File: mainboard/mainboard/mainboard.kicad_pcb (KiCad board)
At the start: 2 copper layers, 100 x 100 mm, 102 parts, among them IC501 SN74HCS138PWR, IC502 SN74HCS138PWR, IC503 SN74HCS138PWR, IC504 SN74HCS138PWR, IC505 SN74HCS151PWR, J1 Barrel_Jack_Switch, J201 Power LED connector, J202 Power button connector, J601 Connector 1, J602 Connector 6, J603 Connector 5, J604 Connector 4, J605 Connector 1, J606 Connector 3, J607 Connector 2, J608 I2C 2, J609 Conn_01x03_Female, J610 Conn_01x03_Female, J611 I2C 1, J612 I2C 3, J801 Micro_SD_Card, U201 RP2040, U301 LD1117S50TR_SOT223, U303 BD9D321EFJ, U304 BD9D321EFJ, U401 W25Q128JVS, U701 hs8836a, Y201 ECS-120-8-36-CGN-TR

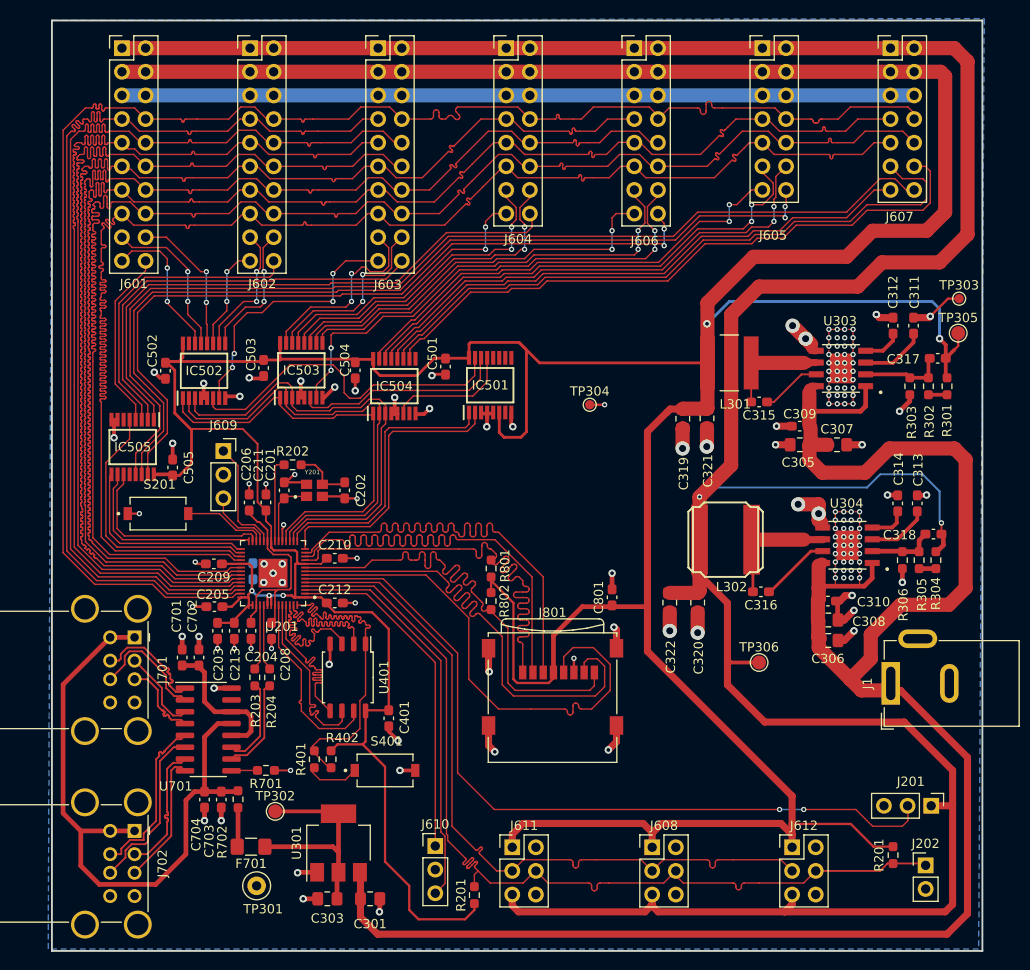
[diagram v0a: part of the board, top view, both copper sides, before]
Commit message: refactored mainboard schematic
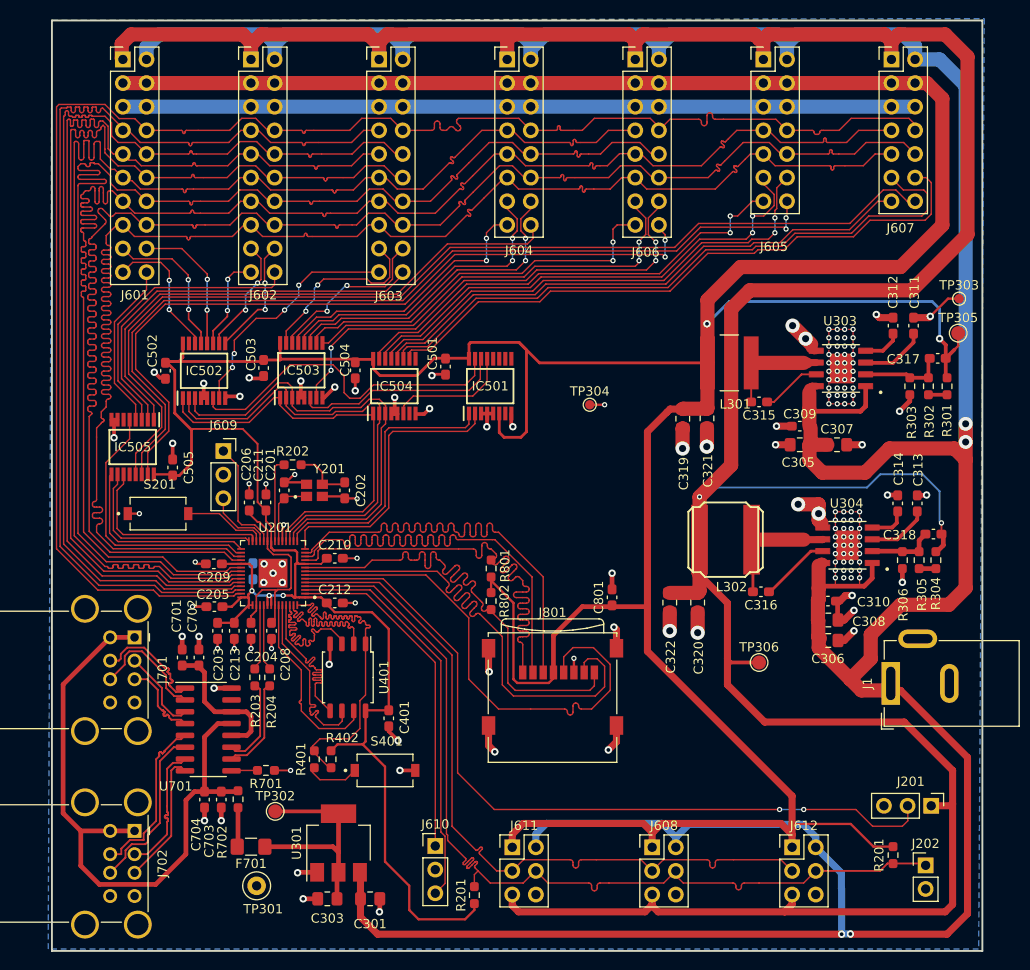
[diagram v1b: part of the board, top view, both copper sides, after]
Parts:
- IC501: value SN74HCS138PWR -> SN74HCS238PWR
- moved J604 1.22 mm to (71.9, 60.2)
- moved J605 1.22 mm to (99.5, 60.2)
- moved J606 1.22 mm to (85.7, 60.2)
- moved J607 1.22 mm to (113.2, 60.2)
- moved J601 1.22 mm to (30.6, 60.2)
- moved J602 1.22 mm to (44.4, 60.2)
- moved J603 1.22 mm to (58.2, 60.2)
- moved IC501 0.10 mm to (70.1, 95.3)
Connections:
- J601 pad 2: +5V_BUS -> VDC
- J602 pad 2: +5V_BUS -> VDC
- J603 pad 2: +5V_BUS -> VDC
- J604 pad 2: +5V_BUS -> VDC
- J605 pad 2: +5V_BUS -> VDC
- J606 pad 2: +5V_BUS -> VDC
- J607 pad 2: +5V_BUS -> VDC
- J608 pad 2: unconnected-(J608-Pin_2) -> VDC
- J611 pad 2: unconnected-(J611-Pin_2) -> VDC
- J612 pad 2: unconnected-(J612-Pin_2) -> VDC
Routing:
- net VDC: track 196.5 -> 393.8 mm, vias 0 -> 4
- net +5V_BUS: track 322.6 -> 345.1 mm
- net /Bus multiplexers & demultiplexers/BUS_CS4: track 28.6 -> 26.2 mm
- net /Bus multiplexers & demultiplexers/BUS_RE2: track 20.3 -> 18.4 mm
- net /Bus multiplexers & demultiplexers/BUS_CS3: track 14.5 -> 12.7 mm
- net /Connectors/BUS.D3: track 142.5 -> 144.3 mm
- net /Bus multiplexers & demultiplexers/BUS_RE1: track 14.6 -> 12.9 mm
- net /Bus multiplexers & demultiplexers/BUS_INT3: track 62.0 -> 60.4 mm
- net /Bus multiplexers & demultiplexers/BUS_INT2: track 45.6 -> 44.0 mm
- net /Bus multiplexers & demultiplexers/BUS_INT1: track 32.8 -> 31.2 mm
- net /Connectors/BUS.D1: track 174.9 -> 176.4 mm
- net /Connectors/BUS.D4: track 109.3 -> 110.8 mm
- net /Connectors/BUS.D5: track 109.2 -> 110.7 mm
- net /Bus multiplexers & demultiplexers/BUS_INT6: track 110.8 -> 109.4 mm
- net +3V3: track 539.0 -> 537.6 mm
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
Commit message: working on new pcb
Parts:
- removed C201, C202: 14p, Capacitor_SMD:C_0603_1608Metric_Pad1.08x0.95mm_HandSolder
- removed C204, C311, C313: 1u, Capacitor_SMD:C_0603_1608Metric_Pad1.08x0.95mm_HandSolder
- removed C206, C208, C209, C210, C211, C212, C213, C309, C310, C315, C316, C401, C501, C502, C503, C504, C505, C702, C704: 100n, Capacitor_SMD:C_0603_1608Metric_Pad1.08x0.95mm_HandSolder
- removed C301: 4.7u, Capacitor_SMD:C_0805_2012Metric_Pad1.18x1.45mm_HandSolder
- removed C303: 10uF, Capacitor_SMD:C_0805_2012Metric_Pad1.18x1.45mm_HandSolder
- removed C305, C306, C307, C308: 10u, Capacitor_SMD:C_0805_2012Metric_Pad1.18x1.45mm_HandSolder
- removed C312, C314: 3300p, Capacitor_SMD:C_0603_1608Metric_Pad1.08x0.95mm_HandSolder
- removed C317, C318: 22p, Capacitor_SMD:C_0603_1608Metric_Pad1.08x0.95mm_HandSolder
- removed C319, C320, C321, C322: 22u, Capacitor_SMD:C_0805_2012Metric_Pad1.18x1.45mm_HandSolder
- removed C701, C703: 4.7u, Capacitor_SMD:C_0603_1608Metric_Pad1.08x0.95mm_HandSolder
- removed C801: 10u, Capacitor_SMD:C_0603_1608Metric_Pad1.08x0.95mm_HandSolder
- removed F701: 500mA, Fuse:Fuse_1206_3216Metric_Pad1.42x1.75mm_HandSolder
- removed IC501: SN74HCS238PWR, footprints:SOP65P640X120-16N
- removed IC502, IC503, IC504: SN74HCS138PWR, footprints:SOP65P640X120-16N
- removed IC505: SN74HCS151PWR, footprints:SOP65P640X120-16N
- removed J201: Power LED connector, Connector_PinHeader_2.54mm:PinHeader_1x03_P2.54mm_Vertical
- removed J202: Power button connector, Connector_PinHeader_2.54mm:PinHeader_1x02_P2.54mm_Vertical
- removed J601: Connector 1, Connector_PinHeader_2.54mm:PinHeader_2x10_P2.54mm_Vertical
- removed J602: Connector 6, Connector_PinHeader_2.54mm:PinHeader_2x10_P2.54mm_Vertical
- removed J603: Connector 5, Connector_PinHeader_2.54mm:PinHeader_2x10_P2.54mm_Vertical
- removed J604: Connector 4, Connector_PinHeader_2.54mm:PinHeader_2x08_P2.54mm_Vertical
- removed J605: Connector 1, Connector_PinHeader_2.54mm:PinHeader_2x07_P2.54mm_Vertical
- removed J606: Connector 3, Connector_PinHeader_2.54mm:PinHeader_2x08_P2.54mm_Vertical
- removed J607: Connector 2, Connector_PinHeader_2.54mm:PinHeader_2x07_P2.54mm_Vertical
- removed J608: I2C 2, Connector_PinHeader_2.54mm:PinHeader_2x03_P2.54mm_Vertical
- removed J609: Conn_01x03_Female, Connector_PinSocket_2.54mm:PinSocket_1x03_P2.54mm_Vertical
- removed J610: Conn_01x03_Female, Connector_PinHeader_2.54mm:PinHeader_1x03_P2.54mm_Vertical
- removed J611: I2C 1, Connector_PinHeader_2.54mm:PinHeader_2x03_P2.54mm_Vertical
- removed J612: I2C 3, Connector_PinHeader_2.54mm:PinHeader_2x03_P2.54mm_Vertical
- removed J701, J702: ~, Connector_USB:USB_A_Wuerth_61400826021_Horizontal_Stacked
- removed J801: Micro_SD_Card, Connector_Card:microSD_HC_Wuerth_693072010801
- removed L301: 2.2u, footprints:IND_NR6028T4R7M
- removed L302: 3.3u, footprints:NRS8030
- removed R201 (x2), R402, R801, R802: 10k, Resistor_SMD:R_0603_1608Metric_Pad0.98x0.95mm_HandSolder
- removed R202, R401: 1k, Resistor_SMD:R_0603_1608Metric_Pad0.98x0.95mm_HandSolder
- removed R203, R204: 27.4R, Resistor_SMD:R_0603_1608Metric_Pad0.98x0.95mm_HandSolder
- removed R301: 68k, Resistor_SMD:R_0603_1608Metric_Pad0.98x0.95mm_HandSolder
- removed R302: 5.6k, Resistor_SMD:R_0603_1608Metric_Pad0.98x0.95mm_HandSolder
- removed R303, R306: 22k, Resistor_SMD:R_0603_1608Metric_Pad0.98x0.95mm_HandSolder
- removed R304: 120k, Resistor_SMD:R_0603_1608Metric_Pad0.98x0.95mm_HandSolder
- removed R305: 3.3k, Resistor_SMD:R_0603_1608Metric_Pad0.98x0.95mm_HandSolder
- removed R701: 100k, Resistor_SMD:R_0603_1608Metric_Pad0.98x0.95mm_HandSolder
- removed R702: 4.7, Resistor_SMD:R_0603_1608Metric_Pad0.98x0.95mm_HandSolder
- removed S201, S401: PTS636_SM43J_SMTR_LFS, footprints:SW_PTS636_SM43J_SMTR_LFS
- removed TP301: TestPoint, TestPoint:TestPoint_Loop_D1.80mm_Drill1.0mm_Beaded
- removed TP302, TP305, TP306: TestPoint, TestPoint:TestPoint_Pad_D1.5mm
- removed TP303, TP304: TestPoint, TestPoint:TestPoint_Pad_D1.0mm
- removed U201: RP2040, footprints:QFN40P700X700X90-57N
- removed U301: LD1117S50TR_SOT223, Package_TO_SOT_SMD:SOT-223-3_TabPin2
- removed U303, U304: BD9D321EFJ, footprints:SOIC127P600X100-9N
- removed U401: W25Q128JVS, Package_SO:SOIC-8_5.23x5.23mm_P1.27mm
- removed U701: hs8836a, Package_SO:SOP-16_3.9x9.9mm_P1.27mm
- removed Y201: ECS-120-8-36-CGN-TR, footprints:XTAL_ECS-120-8-36-CGN-TR
- added C1: 14p, Capacitor_SMD:C_0402_1005Metric_Pad0.74x0.62mm_HandSolder, F.Cu at (65.2, 57.8)
- added C10: 100n, Capacitor_SMD:C_0402_1005Metric_Pad0.74x0.62mm_HandSolder, F.Cu at (68.7, 63.8)
- added C11: 100n, Capacitor_SMD:C_0402_1005Metric_Pad0.74x0.62mm_HandSolder, F.Cu at (66.7, 69.1)
- added C12: 100n, Capacitor_SMD:C_0402_1005Metric_Pad0.74x0.62mm_HandSolder, F.Cu at (62.1, 71.9)
- added C13: 100n, Capacitor_SMD:C_0402_1005Metric_Pad0.74x0.62mm_HandSolder, F.Cu at (56.3, 69.2)
- added C14: 100n, Capacitor_SMD:C_0402_1005Metric_Pad0.74x0.62mm_HandSolder, F.Cu at (61.0, 71.2)
- added C15: 1u, Capacitor_SMD:C_0402_1005Metric_Pad0.74x0.62mm_HandSolder, F.Cu at (245.2, 61.9)
- added C16: 1u, Capacitor_SMD:C_0402_1005Metric_Pad0.74x0.62mm_HandSolder, F.Cu at (254.8, 63.9)
- added C17: 4.7u, Capacitor_SMD:C_0402_1005Metric_Pad0.74x0.62mm_HandSolder, F.Cu at (245.2, 60.0)
- added C18: 100pF, Capacitor_SMD:C_0402_1005Metric_Pad0.74x0.62mm_HandSolder, F.Cu at (245.2, 65.9)
- added C19: 100pF, Capacitor_SMD:C_0402_1005Metric_Pad0.74x0.62mm_HandSolder, F.Cu at (254.8, 65.9)
- added C2: 14p, Capacitor_SMD:C_0402_1005Metric_Pad0.74x0.62mm_HandSolder, F.Cu at (62.3, 54.4)
- added C20: 10uF, Capacitor_SMD:C_0402_1005Metric_Pad0.74x0.62mm_HandSolder, F.Cu at (245.2, 63.9)
- added C21: 2.2u, Capacitor_SMD:C_0402_1005Metric_Pad0.74x0.62mm_HandSolder, F.Cu at (254.8, 61.9)
- added C22: 2.2u, Capacitor_SMD:C_0402_1005Metric_Pad0.74x0.62mm_HandSolder, F.Cu at (254.8, 67.9)
- added C23: 10u, Capacitor_SMD:C_1206_3216Metric_Pad1.33x1.80mm_HandSolder, F.Cu at (134.1, 108.7)
- added C24: 10u, Capacitor_SMD:C_1206_3216Metric_Pad1.33x1.80mm_HandSolder, F.Cu at (117.0, 108.5)
- added C25: 10u, Capacitor_SMD:C_1206_3216Metric_Pad1.33x1.80mm_HandSolder, F.Cu at (131.4, 108.7)
- added C26: 10u, Capacitor_SMD:C_1206_3216Metric_Pad1.33x1.80mm_HandSolder, F.Cu at (114.3, 108.5)
- added C27: 100n, Capacitor_SMD:C_0402_1005Metric_Pad0.74x0.62mm_HandSolder, F.Cu at (136.0, 108.1)
- added C28: 100n, Capacitor_SMD:C_0402_1005Metric_Pad0.74x0.62mm_HandSolder, F.Cu at (118.9, 107.8)
- added C29: 1u, Capacitor_SMD:C_0402_1005Metric_Pad0.74x0.62mm_HandSolder, F.Cu at (144.3, 115.3)
- added C3: 1u, Capacitor_SMD:C_0402_1005Metric_Pad0.74x0.62mm_HandSolder, F.Cu at (58.7, 71.2)
- added C30: 3300p, Capacitor_SMD:C_0402_1005Metric_Pad0.74x0.62mm_HandSolder, F.Cu at (144.3, 114.2)
- added C31: 1u, Capacitor_SMD:C_0402_1005Metric_Pad0.74x0.62mm_HandSolder, F.Cu at (126.9, 115.2)
- added C32: 3300p, Capacitor_SMD:C_0402_1005Metric_Pad0.74x0.62mm_HandSolder, F.Cu at (126.9, 114.1)
- added C33: 100n, Capacitor_SMD:C_0402_1005Metric_Pad0.74x0.62mm_HandSolder, F.Cu at (135.0, 101.9)
- added C34: 100n, Capacitor_SMD:C_0402_1005Metric_Pad0.74x0.62mm_HandSolder, F.Cu at (119.5, 102.5)
- added C35: 22p, Capacitor_SMD:C_0402_1005Metric_Pad0.74x0.62mm_HandSolder, F.Cu at (140.3, 116.5)
- added C36: 22p, Capacitor_SMD:C_0402_1005Metric_Pad0.74x0.62mm_HandSolder, F.Cu at (123.2, 116.3)
- added C37: 22u, Capacitor_SMD:C_1206_3216Metric_Pad1.33x1.80mm_HandSolder, F.Cu at (144.7, 93.6)
- added C38: 22u, Capacitor_SMD:C_1206_3216Metric_Pad1.33x1.80mm_HandSolder, F.Cu at (127.6, 95.2)
- added C39: 22u, Capacitor_SMD:C_1206_3216Metric_Pad1.33x1.80mm_HandSolder, F.Cu at (144.7, 90.9)
- added C4: 100n, Capacitor_SMD:C_0402_1005Metric_Pad0.74x0.62mm_HandSolder, F.Cu at (57.5, 71.2)
- added C40: 22u, Capacitor_SMD:C_1206_3216Metric_Pad1.33x1.80mm_HandSolder, F.Cu at (127.6, 92.6)
- added C41: 4.7u, Capacitor_SMD:C_0402_1005Metric_Pad0.74x0.62mm_HandSolder, F.Cu at (40.0, 121.1)
- added C42: 100n, Capacitor_SMD:C_0402_1005Metric_Pad0.74x0.62mm_HandSolder, F.Cu at (40.0, 123.0)
- added C43: 4.7u, Capacitor_SMD:C_0402_1005Metric_Pad0.74x0.62mm_HandSolder, F.Cu at (40.0, 125.0)
- added C44: 1u, Capacitor_SMD:C_0402_1005Metric_Pad0.74x0.62mm_HandSolder, F.Cu at (60.6, 107.5)
- added C45: 100n, Capacitor_SMD:C_0402_1005Metric_Pad0.74x0.62mm_HandSolder, F.Cu at (70.0, 100.3)
- added C46: 100n, Capacitor_SMD:C_0402_1005Metric_Pad0.74x0.62mm_HandSolder, F.Cu at (69.3, 104.8)
- added C47: 1u, Capacitor_SMD:C_0402_1005Metric_Pad0.74x0.62mm_HandSolder, F.Cu at (61.8, 107.5)
- added C48: 100n, Capacitor_SMD:C_0402_1005Metric_Pad0.74x0.62mm_HandSolder, F.Cu at (58.3, 104.7)
- added C49: 100n, Capacitor_SMD:C_0402_1005Metric_Pad0.74x0.62mm_HandSolder, F.Cu at (66.6, 108.5)
- added C5: 1u, Capacitor_SMD:C_0402_1005Metric_Pad0.74x0.62mm_HandSolder, F.Cu at (59.8, 71.2)
- added C50: 100n, Capacitor_SMD:C_0402_1005Metric_Pad0.74x0.62mm_HandSolder, F.Cu at (65.4, 108.5)
- added C51: 100n, Capacitor_SMD:C_0402_1005Metric_Pad0.74x0.62mm_HandSolder, F.Cu at (62.9, 94.0)
- added C52: 100n, Capacitor_SMD:C_0402_1005Metric_Pad0.74x0.62mm_HandSolder, F.Cu at (63.8, 107.8)
- added C53: 100n, Capacitor_SMD:C_0402_1005Metric_Pad0.74x0.62mm_HandSolder, F.Cu at (64.0, 94.0)
- added C54: 100n, Capacitor_SMD:C_0402_1005Metric_Pad0.74x0.62mm_HandSolder, F.Cu at (58.0, 100.0)
- added C55: 100n, Capacitor_SMD:C_0402_1005Metric_Pad0.74x0.62mm_HandSolder, F.Cu at (59.5, 107.5)
- added C56: 1u, Capacitor_SMD:C_0402_1005Metric_Pad0.74x0.62mm_HandSolder, F.Cu at (232.8, 103.5)
- added C57: 1u, Capacitor_SMD:C_0402_1005Metric_Pad0.74x0.62mm_HandSolder, F.Cu at (232.8, 97.6)
- added C58: 1u, Capacitor_SMD:C_0402_1005Metric_Pad0.74x0.62mm_HandSolder, F.Cu at (236.0, 95.6)
- added C59: 1u, Capacitor_SMD:C_0402_1005Metric_Pad0.74x0.62mm_HandSolder, F.Cu at (239.3, 97.6)
- added C6: 100n, Capacitor_SMD:C_0402_1005Metric_Pad0.74x0.62mm_HandSolder, F.Cu at (61.7, 57.7)
- added C60: 1u, Capacitor_SMD:C_0402_1005Metric_Pad0.74x0.62mm_HandSolder, F.Cu at (232.8, 101.5)
- added C61: 100n, Capacitor_SMD:C_0402_1005Metric_Pad0.74x0.62mm_HandSolder, F.Cu at (239.3, 99.6)
- added C62: 100n, Capacitor_SMD:C_0402_1005Metric_Pad0.74x0.62mm_HandSolder, F.Cu at (232.8, 95.6)
- added C63: 100n, Capacitor_SMD:C_0402_1005Metric_Pad0.74x0.62mm_HandSolder, F.Cu at (232.8, 99.6)
- added C64: 22u, Capacitor_SMD:C_0402_1005Metric_Pad0.74x0.62mm_HandSolder, F.Cu at (236.0, 103.5)
- added C65: 100n, Capacitor_SMD:C_0402_1005Metric_Pad0.74x0.62mm_HandSolder, F.Cu at (239.3, 95.6)
- added C66: 1u, Capacitor_SMD:C_0402_1005Metric_Pad0.74x0.62mm_HandSolder, F.Cu at (236.0, 97.6)
- added C67: 1u, Capacitor_SMD:C_0402_1005Metric_Pad0.74x0.62mm_HandSolder, F.Cu at (236.0, 99.6)
- added C68: 1u, Capacitor_SMD:C_0402_1005Metric_Pad0.74x0.62mm_HandSolder, F.Cu at (236.0, 101.5)
- added C69: 100n, Capacitor_SMD:C_0402_1005Metric_Pad0.74x0.62mm_HandSolder, F.Cu at (110.2, 97.4)
- added C7: 100n, Capacitor_SMD:C_0402_1005Metric_Pad0.74x0.62mm_HandSolder, F.Cu at (63.2, 72.5)
- added C70: 100n, Capacitor_SMD:C_0402_1005Metric_Pad0.74x0.62mm_HandSolder, F.Cu at (102.5, 98.7)
- added C71: 100n, Capacitor_SMD:C_0402_1005Metric_Pad0.74x0.62mm_HandSolder, F.Cu at (87.5, 92.2)
- added C72: 10u, Capacitor_SMD:C_0402_1005Metric_Pad0.74x0.62mm_HandSolder, F.Cu at (306.6, 64.0)
- added C72: 4.7u, Capacitor_SMD:C_0402_1005Metric_Pad0.74x0.62mm_HandSolder, F.Cu at (249.1, 43.9)
- added C73: 14p, Capacitor_SMD:C_0402_1005Metric_Pad0.74x0.62mm_HandSolder, F.Cu at (70.4, 92.8)
- added C73: 100n, Capacitor_SMD:C_0402_1005Metric_Pad0.74x0.62mm_HandSolder, F.Cu at (249.1, 45.8)
- added C74: 4.7u, Capacitor_SMD:C_0402_1005Metric_Pad0.74x0.62mm_HandSolder, F.Cu at (249.1, 47.8)
- added C74: 14p, Capacitor_SMD:C_0402_1005Metric_Pad0.74x0.62mm_HandSolder, F.Cu at (68.2, 90.5)
- added C75: 100n, Capacitor_SMD:C_0402_1005Metric_Pad0.74x0.62mm_HandSolder, F.Cu at (76.8, 113.0)
- added C76: 100n, Capacitor_SMD:C_0402_1005Metric_Pad0.74x0.62mm_HandSolder, F.Cu at (61.1, 81.4)
- added C77: 100n, Capacitor_SMD:C_0402_1005Metric_Pad0.74x0.62mm_HandSolder, F.Cu at (82.3, 77.7)
- added C78: 100n, Capacitor_SMD:C_0402_1005Metric_Pad0.74x0.62mm_HandSolder, F.Cu at (85.7, 85.5)
- added C8: 100n, Capacitor_SMD:C_0402_1005Metric_Pad0.74x0.62mm_HandSolder, F.Cu at (55.6, 63.8)
- added C9: 100n, Capacitor_SMD:C_0402_1005Metric_Pad0.74x0.62mm_HandSolder, F.Cu at (60.6, 57.7)
- added D1: LESD5D5.0CT1G, footprints:TVS_LESD5D5.0CT1G, F.Cu at (24.3, 121.2)
- added D10: LESD5D5.0CT1G, footprints:TVS_LESD5D5.0CT1G, F.Cu at (81.5, 131.1)
- added D10: LESD5D5.0CT1G, footprints:TVS_LESD5D5.0CT1G, F.Cu at (28.2, 128.3)
- added D11: LESD5D5.0CT1G, footprints:TVS_LESD5D5.0CT1G, F.Cu at (63.0, 123.4)
- added D11: WS2812B, LED_SMD:LED_WS2812B_PLCC4_5.0x5.0mm_P3.2mm, F.Cu at (298.4, 90.5)
- added D2: LESD5D5.0CT1G, footprints:TVS_LESD5D5.0CT1G, F.Cu at (59.1, 116.4)
- added D2: LESD5D5.0CT1G, footprints:TVS_LESD5D5.0CT1G, F.Cu at (24.3, 123.6)
- added D3: LESD5D5.0CT1G, footprints:TVS_LESD5D5.0CT1G, F.Cu at (83.1, 131.1)
- added D3: LESD5D5.0CT1G, footprints:TVS_LESD5D5.0CT1G, F.Cu at (24.3, 126.0)
- added D4: LESD5D5.0CT1G, footprints:TVS_LESD5D5.0CT1G, F.Cu at (59.1, 118.7)
- added D4: LESD5D5.0CT1G, footprints:TVS_LESD5D5.0CT1G, F.Cu at (24.3, 128.3)
- added D5: LESD5D5.0CT1G, footprints:TVS_LESD5D5.0CT1G, F.Cu at (24.3, 130.7)
- added D5: LESD5D5.0CT1G, footprints:TVS_LESD5D5.0CT1G, F.Cu at (63.0, 116.4)
- added D6: LESD5D5.0CT1G, footprints:TVS_LESD5D5.0CT1G, F.Cu at (24.3, 133.0)
- added D6: LESD5D5.0CT1G, footprints:TVS_LESD5D5.0CT1G, F.Cu at (59.1, 121.1)
- added D7: LESD5D5.0CT1G, footprints:TVS_LESD5D5.0CT1G, F.Cu at (28.2, 121.2)
- added D7: LESD5D5.0CT1G, footprints:TVS_LESD5D5.0CT1G, F.Cu at (63.0, 118.7)
- added D8: LESD5D5.0CT1G, footprints:TVS_LESD5D5.0CT1G, F.Cu at (59.1, 123.4)
- added D8: LESD5D5.0CT1G, footprints:TVS_LESD5D5.0CT1G, F.Cu at (28.2, 123.6)
- added D9: LESD5D5.0CT1G, footprints:TVS_LESD5D5.0CT1G, F.Cu at (28.2, 126.0)
- added D9: LESD5D5.0CT1G, footprints:TVS_LESD5D5.0CT1G, F.Cu at (63.0, 121.1)
- added IC1: SN74HCS151PWR, footprints:SOP65P640X120-16N, F.Cu at (99.1, 94.6)
- added IC2: SN74HCS151PWR, footprints:SOP65P640X120-16N, F.Cu at (106.7, 94.6)
- added IC3: SN74HCS138PWR, footprints:SOP65P640X120-16N, F.Cu at (91.4, 94.6)
- added IC4: SN74HCS138PWR, footprints:SOP65P640X120-16N, F.Cu at (80.0, 81.3)
- added IC5: SN74HCS138PWR, footprints:SOP65P640X120-16N, F.Cu at (80.0, 87.6)
- added J10: AudioJack4, Connector_Audio:Jack_3.5mm_PJ320D_Horizontal, F.Cu at (103.0, 126.4)
- added J11: AudioJack4, Connector_Audio:Jack_3.5mm_PJ320D_Horizontal, F.Cu at (115.4, 126.4)
- added J12: Conn_01x03_Female, Connector_PinHeader_2.54mm:PinHeader_1x03_P2.54mm_Vertical, F.Cu at (54.4, 54.1)
- added J13: Connector 16-bit, Connector_PinHeader_1.27mm:PinHeader_2x15_P1.27mm_Vertical_SMD, F.Cu at (83.8, 64.1)
- added J14: Connector A 8-bit, Connector_PinHeader_1.27mm:PinHeader_2x10_P1.27mm_Vertical_SMD, F.Cu at (102.2, 79.9)
- added J15: Connector B 8-bit, Connector_PinHeader_1.27mm:PinHeader_2x10_P1.27mm_Vertical_SMD, F.Cu at (102.2, 61.0)
- added J16: Connector A - 4 bit, Connector_PinHeader_1.27mm:PinHeader_2x08_P1.27mm_Vertical_SMD, F.Cu at (120.7, 78.7)
- added J17: Connector B - 4 bit, Connector_PinHeader_1.27mm:PinHeader_2x08_P1.27mm_Vertical_SMD, F.Cu at (120.5, 59.7)
- added J18: Connector A - 2 bit, Connector_PinHeader_1.27mm:PinHeader_2x05_P1.27mm_Vertical_SMD, F.Cu at (139.1, 76.8)
- added J19: Connector B - 2 bit, Connector_PinHeader_1.27mm:PinHeader_2x05_P1.27mm_Vertical_SMD, F.Cu at (139.1, 57.8)
- added J2: ~, Connector_USB:USB_A_Wuerth_61400826021_Horizontal_Stacked, F.Cu at (83.1, 135.0)
- added J3: ~, Connector_USB:USB_A_Wuerth_61400826021_Horizontal_Stacked, F.Cu at (62.9, 135.0)
- added J4: Micro_SD_Card, Connector_Card:microSD_HC_Wuerth_693072010801, F.Cu at (207.6, 139.6)
- added J5: I2C 2, Connector_PinHeader_2.54mm:PinHeader_2x03_P2.54mm_Vertical, F.Cu at (266.5, 61.3)
- added J6: Conn_01x03_Female, Connector_PinSocket_2.54mm:PinSocket_1x03_P2.54mm_Vertical, F.Cu at (58.8, 89.3)
- added J7: I2C 1, Connector_PinHeader_2.54mm:PinHeader_2x03_P2.54mm_Vertical, F.Cu at (273.7, 61.3)
- added J8: I2C 3, Connector_PinHeader_2.54mm:PinHeader_2x03_P2.54mm_Vertical, F.Cu at (280.9, 61.3)
- added J9: Conn_01x03_Female, Connector_PinHeader_2.54mm:PinHeader_1x03_P2.54mm_Vertical, F.Cu at (80.8, 105.7)
- added L1: 3.3u, footprints:NRS8030, F.Cu at (140.5, 99.3)
- added L2: 2.2u, footprints:IND_NR6028T4R7M, F.Cu at (123.6, 100.2)
- added R1: 1k, Resistor_SMD:R_0402_1005Metric_Pad0.72x0.64mm_HandSolder, F.Cu at (62.9, 56.1)
- added R10: 27.4R, Resistor_SMD:R_0402_1005Metric_Pad0.72x0.64mm_HandSolder, F.Cu at (62.3, 110.4)
- added R11: 27.4R, Resistor_SMD:R_0402_1005Metric_Pad0.72x0.64mm_HandSolder, F.Cu at (63.4, 110.4)
- added R12: 1k, Resistor_SMD:R_0402_1005Metric_Pad0.72x0.64mm_HandSolder, F.Cu at (299.2, 78.9)
- added R13: 10k, Resistor_SMD:R_0402_1005Metric_Pad0.72x0.64mm_HandSolder, F.Cu at (306.6, 60.0)
- added R14: 10k, Resistor_SMD:R_0402_1005Metric_Pad0.72x0.64mm_HandSolder, F.Cu at (306.6, 62.0)
- added R15: 1k, Resistor_SMD:R_0402_1005Metric_Pad0.72x0.64mm_HandSolder, F.Cu at (66.1, 92.5)
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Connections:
- net +3V3 renamed +3V3_MCU
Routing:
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- added copper zone on In1.Cu, net GND
- added copper zone on In2.Cu, net GND
- removed copper zone on B.Cu, net GND
- removed copper zone on F.Cu, net GND
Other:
- board size 100 x 100 mm -> 99.2 x 94.1 mm
- copper layers 2 -> 4

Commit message: working on PCB
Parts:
- removed C203: 1u, Capacitor_SMD:C_0402_1005Metric_Pad0.74x0.62mm_HandSolder
- removed C205, C207, C77, C78: 100n, Capacitor_SMD:C_0402_1005Metric_Pad0.74x0.62mm_HandSolder
- removed the C45 at (70.0, 100.3)
- removed the C56 at (232.8, 103.5)
- removed the C66 at (236.0, 97.6)
- removed the C67 at (236.0, 99.6)
- removed the C68 at (236.0, 101.5)
- removed the C69 at (110.2, 97.4)
- removed the C72 at (249.1, 43.9)
- removed C74: 4.7u, Capacitor_SMD:C_0402_1005Metric_Pad0.74x0.62mm_HandSolder
- removed the D10 at (81.5, 131.1)
- removed the D10 at (28.2, 128.3)
- removed the D11 at (63.0, 123.4)
- removed the D2 at (59.1, 116.4)
- removed the D3 at (83.1, 131.1)
- removed the D4 at (59.1, 118.7)
- removed the D5 at (63.0, 116.4)
- removed the D6 at (24.3, 133.0)
- removed the D6 at (59.1, 121.1)
- removed the D7 at (63.0, 118.7)
- removed the D8 at (59.1, 123.4)
- removed the D8 at (28.2, 123.6)
- removed the D9 at (63.0, 121.1)
- removed IC2: SN74HCS151PWR, footprints:SOP65P640X120-16N
- removed IC3, IC4, IC5: SN74HCS138PWR, footprints:SOP65P640X120-16N
- removed J18: Connector A - 2 bit, Connector_PinHeader_1.27mm:PinHeader_2x05_P1.27mm_Vertical_SMD
- removed J19: Connector B - 2 bit, Connector_PinHeader_1.27mm:PinHeader_2x05_P1.27mm_Vertical_SMD
- removed the J7 at (273.7, 61.3)
- removed the R16 at (252.4, 43.9)
- removed S1, S2: PTS636_SM43J_SMTR_LFS, footprints:SW_PTS636_SM43J_SMTR_LFS
- removed the TP1 at (245.9, 88.2)
- added C44: 100n, Capacitor_SMD:C_0402_1005Metric_Pad0.74x0.62mm_HandSolder, F.Cu at (25.5, 105.4)
- added C46: 100n, Capacitor_SMD:C_0402_1005Metric_Pad0.74x0.62mm_HandSolder, F.Cu at (72.1, 101.1)
- added D10: LESD5D5.0CT1G, footprints:TVS_LESD5D5.0CT1G, F.Cu at (77.7, 137.5)
- added D6: LESD5D5.0CT1G, footprints:TVS_LESD5D5.0CT1G, F.Cu at (217.7, 137.9)
- added D8: LESD5D5.0CT1G, footprints:TVS_LESD5D5.0CT1G, F.Cu at (220.1, 137.9)
- added H1: MountingHole, MountingHole:MountingHole_2.2mm_M2_DIN965, F.Cu at (55.0, 130.0)
- added H2: MountingHole, MountingHole:MountingHole_2.2mm_M2_DIN965, F.Cu at (145.0, 130.0)
- added H3: MountingHole, MountingHole:MountingHole_2.2mm_M2_DIN965, F.Cu at (145.0, 55.0)
- added H4: MountingHole, MountingHole:MountingHole_2.2mm_M2_DIN965, F.Cu at (55.0, 55.0)
- added J1: Conn_01x02_Male, Connector_PinHeader_2.54mm:PinHeader_1x02_P2.54mm_Vertical, F.Cu at (59.6, 86.9)
- added R11: 0, Resistor_SMD:R_2512_6332Metric_Pad1.40x3.35mm_HandSolder, F.Cu at (135.9, 92.1)
- added R13: 0, Resistor_SMD:R_2512_6332Metric_Pad1.40x3.35mm_HandSolder, F.Cu at (140.5, 92.1)
- added R14: 0, Resistor_SMD:R_2512_6332Metric_Pad1.40x3.35mm_HandSolder, F.Cu at (128.4, 94.5)
- added R18: 4.7k, Resistor_SMD:R_0603_1608Metric_Pad0.98x0.95mm_HandSolder, F.Cu at (88.6, 101.1)
- added R2: 0, Resistor_SMD:R_1206_3216Metric_Pad1.30x1.75mm_HandSolder, F.Cu at (100.6, 102.0)
- added R21: 1k, Resistor_SMD:R_0402_1005Metric_Pad0.72x0.64mm_HandSolder, F.Cu at (59.4, 91.4)
- added R3: 0, Resistor_SMD:R_1206_3216Metric_Pad1.30x1.75mm_HandSolder, F.Cu at (94.8, 112.1)
- added R4: 0, Resistor_SMD:R_1206_3216Metric_Pad1.30x1.75mm_HandSolder, F.Cu at (113.5, 98.7)
- added TP2: TestPoint, TestPoint:TestPoint_Pad_D1.5mm, F.Cu at (200.8, 91.7)
- added TP3: TestPoint, TestPoint:TestPoint_Pad_D1.5mm, F.Cu at (200.8, 88.2)
- added U10: SN74LVC139APWR, Package_SO:TSSOP-16_4.4x5mm_P0.65mm, F.Cu at (94.7, 81.4)
- added U13: SN74LVC139APWR, Package_SO:TSSOP-16_4.4x5mm_P0.65mm, F.Cu at (75.7, 81.5)
- C57, C58: value 1u -> 100n
- C60: value 1u -> 10u; footprint Capacitor_SMD:C_0402_1005Metric_Pad0.74x0.62mm_HandSolder -> Capacitor_SMD:C_1206_3216Metric_Pad1.33x1.80mm_HandSolder
- C63: value 100n -> 1u
- C64: value 22u -> 47u; footprint Capacitor_SMD:C_0402_1005Metric_Pad0.74x0.62mm_HandSolder -> Capacitor_SMD:C_1206_3216Metric_Pad1.33x1.80mm_HandSolder
- C65: value 100n -> 47u; footprint Capacitor_SMD:C_0402_1005Metric_Pad0.74x0.62mm_HandSolder -> Capacitor_SMD:C_1206_3216Metric_Pad1.33x1.80mm_HandSolder
- C68: renamed from C72; moved to B.Cu
- IC1: footprint footprints:SOP65P640X120-16N -> Package_SO:TSSOP-16_4.4x5mm_P0.65mm
- J13: value Connector 16-bit -> Connector A 16-bit
- J5: value I2C 2 -> Conn_01x02_Male; footprint Connector_PinHeader_2.54mm:PinHeader_2x03_P2.54mm_Vertical -> Connector_PinHeader_2.54mm:PinHeader_1x02_P2.54mm_Vertical
- J6: renamed from J4; moved to B.Cu
- J8: value I2C 3 -> Conn_01x04_Female; footprint Connector_PinHeader_2.54mm:PinHeader_2x03_P2.54mm_Vertical -> Connector_PinHeader_2.54mm:PinHeader_1x04_P2.54mm_Vertical
- R12: value 1k -> 0; footprint Resistor_SMD:R_0402_1005Metric_Pad0.72x0.64mm_HandSolder -> Resistor_SMD:R_2512_6332Metric_Pad1.40x3.35mm_HandSolder
- R17: value 4.7 -> 4.7k; footprint Resistor_SMD:R_0402_1005Metric_Pad0.72x0.64mm_HandSolder -> Resistor_SMD:R_0603_1608Metric_Pad0.98x0.95mm_HandSolder
- R22: renamed from R13; moved to B.Cu
- R23: renamed from R14; moved to B.Cu
- TP4: renamed from TP3; footprint TestPoint:TestPoint_Pad_D1.0mm -> TestPoint:TestPoint_THTPad_D1.5mm_Drill0.7mm
- TP5: renamed from TP4; footprint TestPoint:TestPoint_Pad_D1.0mm -> TestPoint:TestPoint_THTPad_D1.5mm_Drill0.7mm
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- renumbered C22 to C20, C20 to C21, C21 to C22, C44 to C45, C46 to C47, C47 to C48, C48 to C49, C49 to C50, C50 to C51, C51 to C52, C52 to C53, C53 to C54, C54 to C55, C55 to C56, C70 to C66, C71 to C67, C73 to C69, C74 to C70, C75 to C71, C76 to C72, J16 to J15, J17 to J16, J15 to J17, J1 to J2, J2 to J3, J3 to J4, J6 to J7, R7 to R10, R8 to R15, R9 to R16, R10 to R19, R11 to R20, R15 to R24, R16 to R25, R17 to R26, R18 to R27, R2 to R5, R3 to R6, R4 to R7, R5 to R8, R6 to R9, TP2 to TP1, TP5 to TP6, TP6 to TP7, U10 to U11, U11 to U12
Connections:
- C20 pad 1: +3V3_MCU -> Net-(U4-VOUT)
- C21 pad 1: +5V_VBUS -> Net-(U2-VO)
- C22 pad 1: +3V3_SOUTH -> Net-(U3-VOUT)
- C35 pad 1: +5V_BUS -> Net-(C35-Pad1)
- C36 pad 1: +3V3_BUS -> Net-(C36-Pad1)
- C37 pad 1: +5V_BUS -> Net-(C35-Pad1)
- C38 pad 1: +3V3_BUS -> Net-(C36-Pad1)
- C39 pad 1: +5V_BUS -> Net-(C35-Pad1)
- C40 pad 1: +3V3_BUS -> Net-(C36-Pad1)
- C41 pad 1: +3V3_SOUTH -> +3V3_USB_HUB
- C42 pad 1: +3V3_SOUTH -> +3V3_USB_HUB
- C57 pad 1: Net-(U9-AVDD) -> /South Bridge/Audio DAC/AUX_IN.L
- C57 pad 2: GND -> Net-(U9-INL)
- C59 pad 1: +3V3_SOUTH -> Net-(U9-AVDD)
- C60 pad 1: Net-(U9-AVDD) -> +3V3_SOUTH
- C61 pad 1: +3V3_SOUTH -> Net-(U9-AVDD)
- C62 pad 1: Net-(U9-AVDD) -> +3V3_SOUTH
- C63 pad 1: Net-(U9-AVDD) -> Net-(U9-REF)
- C64 pad 1: +3V3_SOUTH -> Net-(U9-HPR)
- C64 pad 2: GND -> /South Bridge/Audio DAC/AUDIO_OUT.R
- C65 pad 1: +3V3_SOUTH -> Net-(U9-HPL)
- C65 pad 2: GND -> /South Bridge/Audio DAC/AUDIO_OUT.L
- C66 pad 1: +3V3_MCU -> +3V3_SOUTH
- C67 pad 1: +3V3_MCU -> +3V3_SOUTH
- IC1 pad 1: /RP2040 Core/BUS_DET.IN1 -> /RP2040 Core/BUS_DET.IN2
- IC1 pad 12: /RP2040 Core/BUS_DET.IN3 -> /RP2040 Core/BUS_DET.IN4
- IC1 pad 13: /RP2040 Core/BUS_INT.IN3 -> /RP2040 Core/BUS_INT.IN2
- IC1 pad 14: /RP2040 Core/BUS_DET.IN2 -> /RP2040 Core/BUS_INT.IN1
- IC1 pad 15: /RP2040 Core/BUS_INT.IN2 -> /RP2040 Core/BUS_DET.IN3
- IC1 pad 16: +3V3_MCU -> +3V3_SOUTH
- IC1 pad 2: /RP2040 Core/BUS_INT.IN1 -> /RP2040 Core/BUS_DET.IN1
- IC1 pad 5: /South Bridge/BUS_INT.OUT -> /South Bridge/BUS_DET_OUT
- J13 pad 1: +5V_BUS -> GND
- J13 pad 10: /RP2040 Core/MCU Connectors/BUS_NORTH.D13 -> /RP2040 Core/MCU Connectors/BUS_NORTH.D8
- J13 pad 11: /RP2040 Core/MCU Connectors/BUS_NORTH.D12 -> /RP2040 Core/MCU Connectors/BUS_NORTH.D7
- J13 pad 12: /RP2040 Core/MCU Connectors/BUS_NORTH.D11 -> /RP2040 Core/MCU Connectors/BUS_NORTH.D6
- J13 pad 13: /RP2040 Core/MCU Connectors/BUS_NORTH.D10 -> /RP2040 Core/MCU Connectors/BUS_NORTH.D5
- J13 pad 14: /RP2040 Core/MCU Connectors/BUS_NORTH.D9 -> /RP2040 Core/MCU Connectors/BUS_NORTH.D4
- J13 pad 15: /RP2040 Core/MCU Connectors/BUS_NORTH.D8 -> /RP2040 Core/MCU Connectors/BUS_NORTH.D3
- J13 pad 16: /RP2040 Core/MCU Connectors/BUS_NORTH.D7 -> /RP2040 Core/MCU Connectors/BUS_NORTH.D2
- J13 pad 17: /RP2040 Core/MCU Connectors/BUS_NORTH.D6 -> /RP2040 Core/MCU Connectors/BUS_NORTH.D1
- J13 pad 18: /RP2040 Core/MCU Connectors/BUS_NORTH.D5 -> /RP2040 Core/MCU Connectors/BUS_NORTH.D0
- J13 pad 19: /RP2040 Core/MCU Connectors/BUS_NORTH.D4 -> /RP2040 Core/MCU Connectors/BUS_NORTH.RWDS
- J13 pad 2: +5V_BUS -> GND
- J13 pad 20: /RP2040 Core/MCU Connectors/BUS_NORTH.D3 -> /RP2040 Core/MCU Connectors/BUS_NORTH.CLK1
- J13 pad 21: /RP2040 Core/MCU Connectors/BUS_NORTH.D2 -> /RP2040 Core/MCU Connectors/BUS_CS#A0
- J13 pad 22: /RP2040 Core/MCU Connectors/BUS_NORTH.D1 -> /RP2040 Core/MCU Connectors/BUS_CS#A1
- J13 pad 23: /RP2040 Core/MCU Connectors/BUS_NORTH.D0 -> /RP2040 Core/BUS_DET.IN0
- J13 pad 24: /RP2040 Core/MCU Connectors/BUS_NORTH.CLK1 -> /RP2040 Core/BUS_RE#.OUT0
- J13 pad 25: /RP2040 Core/MCU Connectors/BUS_CS#A0 -> /RP2040 Core/BUS_INT.IN0
- J13 pad 26: /RP2040 Core/MCU Connectors/BUS_CS#A1 -> +5V_BUS
- J13 pad 27: /RP2040 Core/BUS_RE#.OUT0 -> +3V3_BUS
- J13 pad 28: /RP2040 Core/BUS_DET.IN0 -> GND
- J13 pad 29: /RP2040 Core/BUS_INT.IN0 -> GND
- J13 pad 3: +3V3_BUS -> /RP2040 Core/MCU Connectors/BUS_NORTH.D15
- J13 pad 4: +3V3_BUS -> /RP2040 Core/MCU Connectors/BUS_NORTH.D14
- J13 pad 5: GND -> /RP2040 Core/MCU Connectors/BUS_NORTH.D13
- J13 pad 6: GND -> /RP2040 Core/MCU Connectors/BUS_NORTH.D12
- J13 pad 7: /RP2040 Core/MCU Connectors/BUS_NORTH.RWDS -> /RP2040 Core/MCU Connectors/BUS_NORTH.D11
- J13 pad 8: /RP2040 Core/MCU Connectors/BUS_NORTH.D15 -> /RP2040 Core/MCU Connectors/BUS_NORTH.D10
- J13 pad 9: /RP2040 Core/MCU Connectors/BUS_NORTH.D14 -> /RP2040 Core/MCU Connectors/BUS_NORTH.D9
- J14 pad 1: +3V3_BUS -> /RP2040 Core/MCU Connectors/BUS_NORTH.D15
- J14 pad 10: /RP2040 Core/MCU Connectors/BUS_NORTH.D3 -> /RP2040 Core/MCU Connectors/BUS_NORTH.CLK1
- J14 pad 11: /RP2040 Core/MCU Connectors/BUS_NORTH.D2 -> /RP2040 Core/MCU Connectors/BUS_CS#A2
- J14 pad 12: /RP2040 Core/MCU Connectors/BUS_NORTH.D1 -> unconnected-(J14-Pin_12)
- J14 pad 13: /RP2040 Core/MCU Connectors/BUS_NORTH.D0 -> /RP2040 Core/BUS_DET.IN1
- J14 pad 14: /RP2040 Core/MCU Connectors/BUS_NORTH.CLK1 -> /RP2040 Core/BUS_RE#.OUT1
- J14 pad 15: /RP2040 Core/MCU Connectors/BUS_CS#A2 -> unconnected-(J14-Pin_15)
- J14 pad 16: /RP2040 Core/MCU Connectors/BUS_CS#A3 -> +5V_BUS
- J14 pad 17: /RP2040 Core/BUS_RE#.OUT4 -> +3V3_BUS
- J14 pad 18: /RP2040 Core/BUS_DET.IN4 -> GND
- J14 pad 19: /RP2040 Core/BUS_INT.IN4 -> GND
- J14 pad 2: +5V_BUS -> /RP2040 Core/MCU Connectors/BUS_NORTH.D14
- J14 pad 3: GND -> /RP2040 Core/MCU Connectors/BUS_NORTH.D13
- J14 pad 4: GND -> /RP2040 Core/MCU Connectors/BUS_NORTH.D12
- J14 pad 5: /RP2040 Core/MCU Connectors/BUS_NORTH.RWDS -> /RP2040 Core/MCU Connectors/BUS_NORTH.D11
- J14 pad 6: /RP2040 Core/MCU Connectors/BUS_NORTH.D7 -> /RP2040 Core/MCU Connectors/BUS_NORTH.D10
- J14 pad 7: /RP2040 Core/MCU Connectors/BUS_NORTH.D6 -> /RP2040 Core/MCU Connectors/BUS_NORTH.D9
- J14 pad 8: /RP2040 Core/MCU Connectors/BUS_NORTH.D5 -> /RP2040 Core/MCU Connectors/BUS_NORTH.D8
- J14 pad 9: /RP2040 Core/MCU Connectors/BUS_NORTH.D4 -> /RP2040 Core/MCU Connectors/BUS_NORTH.RWDS
- J15 pad 1: +3V3_BUS -> /RP2040 Core/MCU Connectors/BUS_NORTH.D11
- J15 pad 10: /RP2040 Core/MCU Connectors/BUS_NORTH.CLK1 -> /RP2040 Core/BUS_RE#.OUT2
- J15 pad 11: /RP2040 Core/MCU Connectors/BUS_CS#A4 -> unconnected-(J15-Pin_11)
- J15 pad 12: /RP2040 Core/MCU Connectors/BUS_CS#A5 -> +5V_BUS
- J15 pad 13: /RP2040 Core/BUS_RE#.OUT5 -> +3V3_BUS
- J15 pad 14: /RP2040 Core/BUS_DET.IN5 -> GND
- J15 pad 15: /RP2040 Core/BUS_INT.IN5 -> GND
- J15 pad 2: +5V_BUS -> /RP2040 Core/MCU Connectors/BUS_NORTH.D10
- J15 pad 3: GND -> /RP2040 Core/MCU Connectors/BUS_NORTH.D9
- J15 pad 4: GND -> /RP2040 Core/MCU Connectors/BUS_NORTH.D8
- J15 pad 6: /RP2040 Core/MCU Connectors/BUS_NORTH.D7 -> /RP2040 Core/MCU Connectors/BUS_NORTH.CLK1
- J15 pad 7: /RP2040 Core/MCU Connectors/BUS_NORTH.D6 -> /RP2040 Core/MCU Connectors/BUS_CS#A3
- J15 pad 8: /RP2040 Core/MCU Connectors/BUS_NORTH.D5 -> unconnected-(J15-Pin_8)
- J15 pad 9: /RP2040 Core/MCU Connectors/BUS_NORTH.D4 -> /RP2040 Core/BUS_DET.IN2
- J16 pad 1: +3V3_BUS -> /RP2040 Core/MCU Connectors/BUS_NORTH.D3
- J16 pad 10: /RP2040 Core/MCU Connectors/BUS_NORTH.CLK0 -> /RP2040 Core/BUS_RE#.OUT4
- J16 pad 11: /RP2040 Core/MCU Connectors/BUS_CS#B4 -> /RP2040 Core/BUS_INT.IN2
- J16 pad 12: /RP2040 Core/MCU Connectors/BUS_CS#B5 -> +5V_BUS
- J16 pad 13: /RP2040 Core/BUS_RE#.OUT2 -> +3V3_BUS
- J16 pad 14: /RP2040 Core/BUS_DET.IN2 -> GND
- J16 pad 15: /RP2040 Core/BUS_INT.IN2 -> GND
- J16 pad 2: +5V_BUS -> /RP2040 Core/MCU Connectors/BUS_NORTH.D2
- J16 pad 3: GND -> /RP2040 Core/MCU Connectors/BUS_NORTH.D1
- J16 pad 4: GND -> /RP2040 Core/MCU Connectors/BUS_NORTH.D0
- J16 pad 6: /RP2040 Core/MCU Connectors/BUS_NORTH.D15 -> /RP2040 Core/MCU Connectors/BUS_NORTH.CLK0
- J16 pad 7: /RP2040 Core/MCU Connectors/BUS_NORTH.D14 -> /RP2040 Core/MCU Connectors/BUS_CS#B2
- J16 pad 8: /RP2040 Core/MCU Connectors/BUS_NORTH.D13 -> /RP2040 Core/MCU Connectors/BUS_CS#B3
- J16 pad 9: /RP2040 Core/MCU Connectors/BUS_NORTH.D12 -> /RP2040 Core/BUS_DET.IN4
- J17 pad 1: +3V3_BUS -> /RP2040 Core/MCU Connectors/BUS_NORTH.D7
- J17 pad 10: /RP2040 Core/MCU Connectors/BUS_NORTH.D11 -> /RP2040 Core/MCU Connectors/BUS_NORTH.CLK0
- J17 pad 11: /RP2040 Core/MCU Connectors/BUS_NORTH.D10 -> /RP2040 Core/MCU Connectors/BUS_CS#B0
- J17 pad 12: /RP2040 Core/MCU Connectors/BUS_NORTH.D9 -> /RP2040 Core/MCU Connectors/BUS_CS#B1
- J17 pad 13: /RP2040 Core/MCU Connectors/BUS_NORTH.D8 -> /RP2040 Core/BUS_DET.IN3
- J17 pad 14: /RP2040 Core/MCU Connectors/BUS_NORTH.CLK0 -> /RP2040 Core/BUS_RE#.OUT3
- J17 pad 15: /RP2040 Core/MCU Connectors/BUS_CS#B2 -> /RP2040 Core/BUS_INT.IN1
- J17 pad 16: /RP2040 Core/MCU Connectors/BUS_CS#B3 -> +5V_BUS
- J17 pad 17: /RP2040 Core/BUS_RE#.OUT1 -> +3V3_BUS
- J17 pad 18: /RP2040 Core/BUS_DET.IN1 -> GND
- J17 pad 19: /RP2040 Core/BUS_INT.IN1 -> GND
- J17 pad 2: +5V_BUS -> /RP2040 Core/MCU Connectors/BUS_NORTH.D6
- J17 pad 3: GND -> /RP2040 Core/MCU Connectors/BUS_NORTH.D5
- J17 pad 4: GND -> /RP2040 Core/MCU Connectors/BUS_NORTH.D4
- J17 pad 5: /RP2040 Core/MCU Connectors/BUS_NORTH.RWDS -> /RP2040 Core/MCU Connectors/BUS_NORTH.D3
- J17 pad 6: /RP2040 Core/MCU Connectors/BUS_NORTH.D15 -> /RP2040 Core/MCU Connectors/BUS_NORTH.D2
- J17 pad 7: /RP2040 Core/MCU Connectors/BUS_NORTH.D14 -> /RP2040 Core/MCU Connectors/BUS_NORTH.D1
- J17 pad 8: /RP2040 Core/MCU Connectors/BUS_NORTH.D13 -> /RP2040 Core/MCU Connectors/BUS_NORTH.D0
- J17 pad 9: /RP2040 Core/MCU Connectors/BUS_NORTH.D12 -> /RP2040 Core/MCU Connectors/BUS_NORTH.RWDS
- J5 pad 1: +3V3_BUS -> Net-(J5-Pin_1)
- J5 pad 2: unconnected-(J5-Pin_2) -> /South Bridge/POWER_BUTTON
- J8 pad 2: unconnected-(J8-Pin_2) -> GND
- J8 pad 3: /South Bridge/Audio DAC/I2C.SCL -> /South Bridge/Audio DAC/I2C.SDA
- J8 pad 4: /South Bridge/Audio DAC/I2C.SDA -> /South Bridge/Audio DAC/I2C.SCL
- L1 pad 2: +5V_BUS -> Net-(C35-Pad1)
- L2 pad 2: +3V3_BUS -> Net-(C36-Pad1)
- R12 pad 1: Net-(R12-Pad1) -> +3V3_BUS
- R12 pad 2: +3V3_SOUTH -> Net-(C36-Pad1)
- R17 pad 1: Net-(U10-VCC) -> /South Bridge/Audio DAC/I2C.SCL
- R17 pad 2: +5V_VBUS -> +3V3_SOUTH
- R5 pad 1: +5V_BUS -> Net-(C35-Pad1)
- R8 pad 1: +3V3_BUS -> Net-(C36-Pad1)
- TP1 pad 1: +5V_VBUS -> Net-(U2-VO)
- TP6 pad 1: +5V_BUS -> Net-(C35-Pad1)
- TP7 pad 1: +3V3_BUS -> Net-(C36-Pad1)
- U1 pad 11: /RP2040 Core/MCU Connectors/BUS_NORTH.D6 -> /RP2040 Core/MCU Connectors/BUS_NORTH.D5
- U1 pad 12: /RP2040 Core/MCU Connectors/BUS_NORTH.D7 -> /RP2040 Core/MCU Connectors/BUS_NORTH.D6
- U1 pad 13: /RP2040 Core/MCU Connectors/BUS_NORTH.D8 -> /RP2040 Core/MCU Connectors/BUS_NORTH.D7
- U1 pad 14: /RP2040 Core/MCU Connectors/BUS_NORTH.D9 -> /RP2040 Core/MCU Connectors/BUS_NORTH.D8
- U1 pad 15: /RP2040 Core/MCU Connectors/BUS_NORTH.D10 -> /RP2040 Core/MCU Connectors/BUS_NORTH.D9
- U1 pad 16: /RP2040 Core/MCU Connectors/BUS_NORTH.D11 -> /RP2040 Core/MCU Connectors/BUS_NORTH.D10
- U1 pad 17: /RP2040 Core/MCU Connectors/BUS_NORTH.D12 -> /RP2040 Core/MCU Connectors/BUS_NORTH.D11
- U1 pad 18: /RP2040 Core/MCU Connectors/BUS_NORTH.D13 -> /RP2040 Core/MCU Connectors/BUS_NORTH.D12
- U1 pad 27: /RP2040 Core/MCU Connectors/BUS_NORTH.D14 -> /RP2040 Core/MCU Connectors/BUS_NORTH.D13
- U1 pad 28: /RP2040 Core/MCU Connectors/BUS_NORTH.D15 -> /RP2040 Core/MCU Connectors/BUS_NORTH.D14
- U1 pad 29: /RP2040 Core/MCU Connectors/BUS_NORTH.RWDS -> /RP2040 Core/MCU Connectors/BUS_NORTH.D15
- U1 pad 30: unconnected-(U1-GPIO19) -> /RP2040 Core/BUS_SOUTH.D0
- U1 pad 31: /RP2040 Core/BUS_SOUTH.CLK -> /RP2040 Core/BUS_SOUTH.D1
- U1 pad 32: /RP2040 Core/BUS_SOUTH.D0 -> /RP2040 Core/BUS_SOUTH.D2
- U1 pad 34: /RP2040 Core/BUS_SOUTH.D1 -> /RP2040 Core/BUS_SOUTH.D3
- U1 pad 35: /RP2040 Core/BUS_SOUTH.D2 -> /RP2040 Core/BUS_SOUTH.CLK
- U1 pad 36: /RP2040 Core/BUS_SOUTH.D3 -> /RP2040 Core/North Bridge BUS multiplexer/BUS_CTRL.CS#3
- U1 pad 37: /RP2040 Core/North Bridge BUS multiplexer/BUS_CTRL.CS#B_EN -> /RP2040 Core/North Bridge BUS multiplexer/BUS_CTRL.CS#2
- U1 pad 38: /RP2040 Core/North Bridge BUS multiplexer/BUS_CTRL.CS#2 -> /RP2040 Core/North Bridge BUS multiplexer/BUS_CTRL.CS#B_EN
- U1 pad 39: /RP2040 Core/North Bridge BUS multiplexer/BUS_CTRL.CS#1 -> /RP2040 Core/North Bridge BUS multiplexer/BUS_CTRL.CS#A_EN
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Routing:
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- added copper zone on F.Cu, net +3V3_BUS
- added copper zone on F.Cu, net +3V3_MCU
- added copper zone on F.Cu, net +5V_BUS
- added copper zone on F.Cu, net GND
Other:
- board size 99.2 x 94.1 mm -> 100 x 100 mm
- board text added: "J2"
